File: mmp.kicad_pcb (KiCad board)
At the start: 2 copper layers, 49.2 x 102.3 mm, 26 parts, among them J2 Conn_01x06_Socket, SW1 SW_Push, SW10 SW_Push, SW11 SW_Push, SW12 SW_Push, SW2 SW_Push, SW3 SW_Push, SW4 SW_Push, SW5 SW_Push, SW6 SW_Push, SW7 SW_Push, SW8 SW_Push, SW9 SW_Push, U1 ADAFRUIT_QT_PY

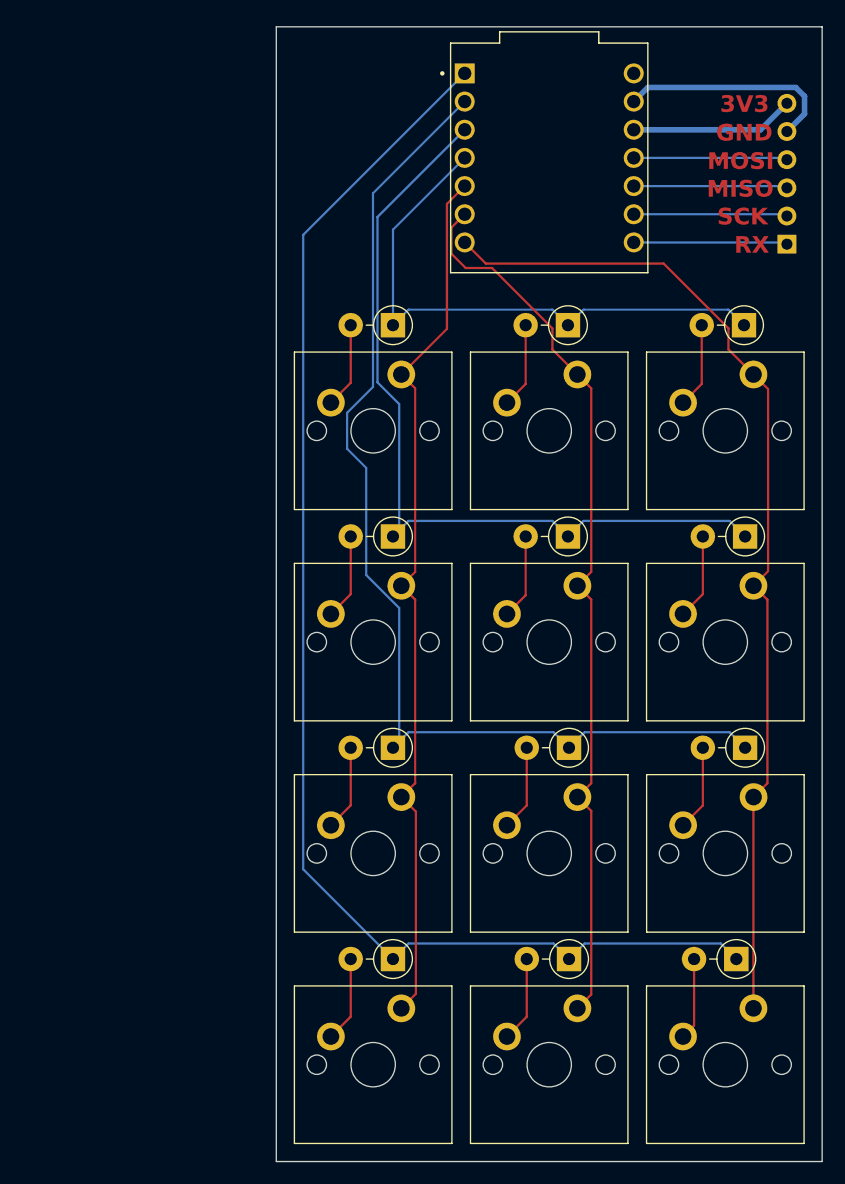
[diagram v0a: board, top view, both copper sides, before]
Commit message: Better pcb layout
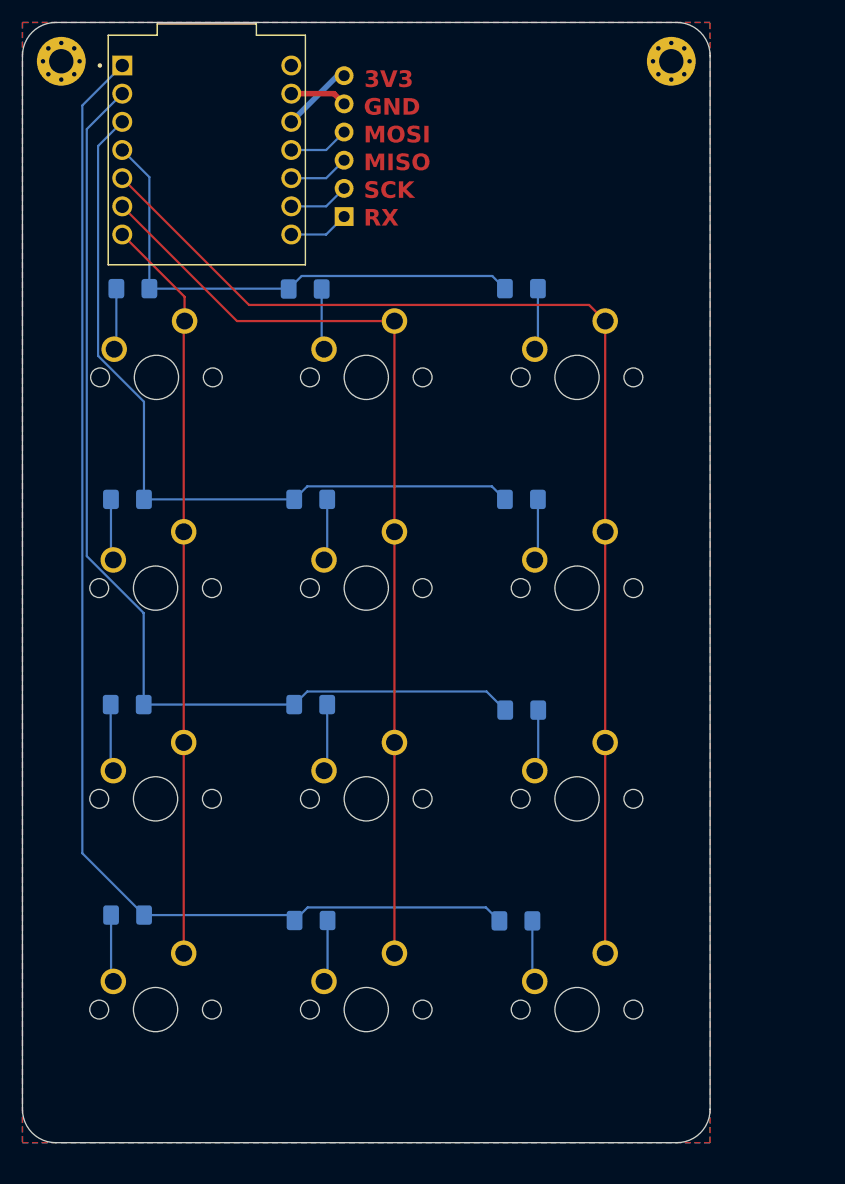
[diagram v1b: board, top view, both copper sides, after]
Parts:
- added REF**: MountingHole_2.2mm_M2_Pad_Via, MountingHole:MountingHole_2.2mm_M2_Pad_Via, F.Cu at (151.5, 40.5)
- added REF**: MountingHole_2.2mm_M2_Pad_Via, MountingHole:MountingHole_2.2mm_M2_Pad_Via, F.Cu at (96.5, 40.5)
- D1, D10, D11, D12, D2, D3, D4, D5, D6, D7, D8, D9: footprint Diode_THT:D_DO-41_SOD81_P3.81mm_Vertical_AnodeUp -> Diode_SMD:D_1206_3216Metric_Pad1.42x1.75mm_HandSolder; moved to B.Cu
- SW1, SW10, SW11, SW12, SW2, SW3, SW4, SW5, SW6, SW7, SW8, SW9: footprint PCM_Switch_Keyboard_Cherry_MX:SW_Cherry_MX_PCB -> mx_solderable:MX-Solderable-1U
- moved J2 40.0 mm to (122.0, 54.5)
- moved U1 30.9 mm to (109.6, 48.5)
- moved D7 24.3 mm to (102.4, 98.5)
- moved D10 24.3 mm to (102.5, 117.5)
- moved D4 24.2 mm to (102.5, 80.0)
- moved D2 23.9 mm to (118.5, 61.0), turned to 0 degrees
- moved D1 23.7 mm to (103.0, 61.0)
- moved D8 23.6 mm to (119.0, 98.5), turned to 0 degrees
- moved D11 23.5 mm to (119.0, 118.0), turned to 0 degrees
- moved D5 23.4 mm to (119.0, 80.0), turned to 0 degrees
- moved D6 20.4 mm to (138.0, 80.0), turned to 0 degrees
- moved D9 20.4 mm to (138.0, 99.0), turned to 0 degrees
- moved D3 20.3 mm to (138.0, 61.0), turned to 0 degrees
- moved SW10 20.2 mm to (105.0, 126.0)
- moved SW7 20.2 mm to (105.0, 107.0)
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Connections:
- U1 pad 5: /col0 -> /col2
- U1 pad 7: /col2 -> /col0
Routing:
- net GND: track 20.1 -> 5.14 mm
- net /col2: track 91.4 -> 105.9 mm
- net /col0: track 79.7 -> 67.2 mm
- net /row3: track 122.5 -> 113.6 mm
- net /ext2: track 13.9 -> 5.43 mm
- net /ext1: track 13.9 -> 5.43 mm
- net /ext0: track 13.9 -> 5.43 mm
- net /ext3: track 13.9 -> 5.43 mm
- net +3.3V: track 14.8 -> 6.48 mm
- net /row2: track 98.9 -> 92.3 mm
- net /row0: track 51.7 -> 46.5 mm
- net /row1: track 75.0 -> 70.2 mm
- net /col1: track 81.3 -> 85.8 mm
- net Net-(D1-A): track 7.73 -> 5.54 mm
- net Net-(D4-A): track 7.73 -> 5.55 mm
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- added copper zone on B.Cu, net GND
- added copper zone on F.Cu, net GND
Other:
- board size 49.2 x 102.3 mm -> 62 x 101 mm
